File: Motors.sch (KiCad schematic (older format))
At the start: 23 parts, among them J10 Screw_Terminal_01x02, J11 Screw_Terminal_01x02, J12 Screw_Terminal_01x02, J2 MOTOR_1, J3 MOTOR_2, J7 MOTOR_3, J8 MOTOR_4, J9 Screw_Terminal_01x02, U10 TXB0104D, U11 VNH5019, U3 VNH5019, U4 VNH5019, U8 TXB0104D, U9 VNH5019

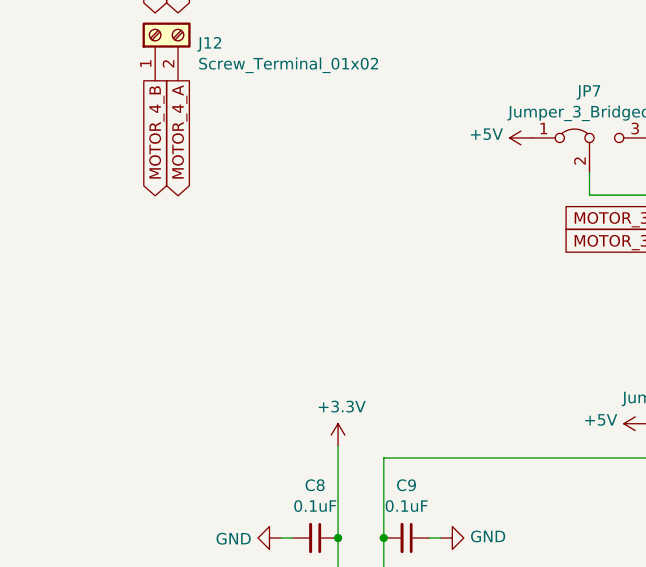
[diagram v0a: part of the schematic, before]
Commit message: Rev B
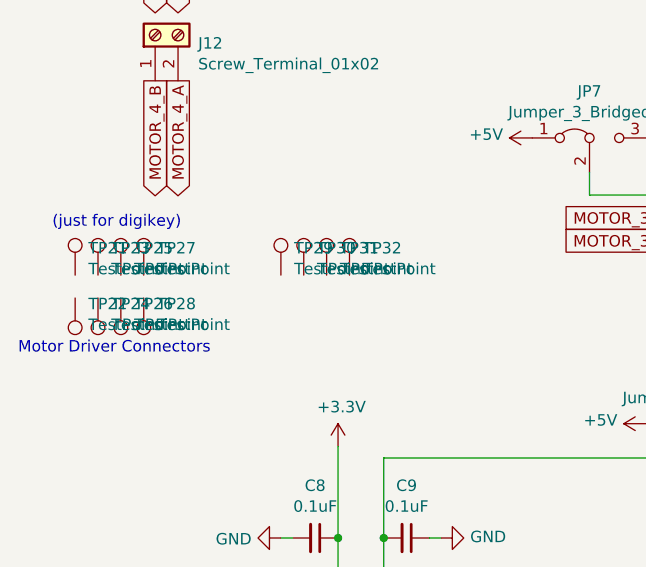
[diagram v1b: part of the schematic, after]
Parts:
- added TP21, TP22, TP23, TP24, TP25, TP26, TP27, TP28, TP29, TP30, TP31, TP32: TestPoint, symbol Connector:TestPoint
- C10, C11, C8, C9: DigiKey (none) -> 399-1100-1-ND
- J10, J11, J12, J9: DigiKey (none) -> 277-1247-ND
- U10, U8: DigiKey (none) -> 296-21928-1-ND
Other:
- note added: "(just for digikey)"
- note added: "Motor Driver Connectors"
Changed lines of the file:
@@
 F 2 "Package_SO:SOIC-14_3.9x8.7mm_P1.27mm" H 2100 5750 50  0001 C CNN
 F 3 "http://www.ti.com/lit/ds/symlink/txb0104.pdf" H 2210 6595 50  0001 C CNN
+F 4 "296-21928-1-ND" H 2100 6500 50  0001 C CNN "DigiKey"
 	1    2100 6500
 	1    0    0    -1
@@
 F 2 "Capacitor_SMD:C_0603_1608Metric_Pad1.05x0.95mm_HandSolder" H 1900 5650 50  0001 C CNN
 F 3 "~" H 1900 5650 50  0001 C CNN
+F 4 "399-1100-1-ND" H 1900 5650 50  0001 C CNN "DigiKey"
 	1    1900 5650
 	0    1    1    0
@@
 F 2 "Capacitor_SMD:C_0603_1608Metric_Pad1.05x0.95mm_HandSolder" H 2300 5650 50  0001 C CNN
 F 3 "~" H 2300 5650 50  0001 C CNN
+F 4 "399-1100-1-ND" H 2300 5650 50  0001 C CNN "DigiKey"
 	1    2300 5650
 	0    1    1    0
@@
 F 2 "Package_SO:SOIC-14_3.9x8.7mm_P1.27mm" H 5050 5750 50  0001 C CNN
 F 3 "http://www.ti.com/lit/ds/symlink/txb0104.pdf" H 5160 6595 50  0001 C CNN
+F 4 "296-21928-1-ND" H 5050 6500 50  0001 C CNN "DigiKey"
 	1    5050 6500
 	1    0    0    -1
@@
 F 2 "Capacitor_SMD:C_0603_1608Metric_Pad1.05x0.95mm_HandSolder" H 4850 5650 50  0001 C CNN
 F 3 "~" H 4850 5650 50  0001 C CNN
+F 4 "399-1100-1-ND" H 4850 5650 50  0001 C CNN "DigiKey"
 	1    4850 5650
 	0    1    1    0
@@
 F 2 "Capacitor_SMD:C_0603_1608Metric_Pad1.05x0.95mm_HandSolder" H 5250 5650 50  0001 C CNN
 F 3 "~" H 5250 5650 50  0001 C CNN
+F 4 "399-1100-1-ND" H 5250 5650 50  0001 C CNN "DigiKey"
 	1    5250 5650
 	0    1    1    0
@@
 F 2 "TerminalBlock_Phoenix:TerminalBlock_Phoenix_MKDS-3-2-5.08_1x02_P5.08mm_Horizontal" H 1200 1050 50  0001 C CNN
 F 3 "~" H 1200 1050 50  0001 C CNN
+F 4 "277-1247-ND" H 1200 1050 50  0001 C CNN "DigiKey"
 	1    1200 1050
 	0    -1   -1   0
@@
 F 2 "TerminalBlock_Phoenix:TerminalBlock_Phoenix_MKDS-3-2-5.08_1x02_P5.08mm_Horizontal" H 1200 1850 50  0001 C CNN
 F 3 "~" H 1200 1850 50  0001 C CNN
+F 4 "277-1247-ND" H 1200 1850 50  0001 C CNN "DigiKey"
 	1    1200 1850
 	0    -1   -1   0
@@
 F 2 "TerminalBlock_Phoenix:TerminalBlock_Phoenix_MKDS-3-2-5.08_1x02_P5.08mm_Horizontal" H 1200 2650 50  0001 C CNN
 F 3 "~" H 1200 2650 50  0001 C CNN
+F 4 "277-1247-ND" H 1200 2650 50  0001 C CNN "DigiKey"
 	1    1200 2650
 	0    -1   -1   0
@@
 F 2 "TerminalBlock_Phoenix:TerminalBlock_Phoenix_MKDS-3-2-5.08_1x02_P5.08mm_Horizontal" H 1200 3450 50  0001 C CNN
 F 3 "~" H 1200 3450 50  0001 C CNN
+F 4 "277-1247-ND" H 1200 3450 50  0001 C CNN "DigiKey"
 	1    1200 3450
 	0    -1   -1   0
@@
 Wire Wire Line
 	2200 5300 2200 5650
+$Comp
+L Connector:TestPoint TP21
+U 1 1 5EF090F9
+P 850 4500
+F 0 "TP21" H 908 4618 50  0000 L CNN
+F 1 "TestPoint" H 908 4527 50  0000 L CNN
+F 2 "" H 1050 4500 50  0001 C CNN
+F 3 "~" H 1050 4500 50  0001 C CNN
+F 4 "S7043-ND" H 850 4500 50  0001 C CNN "DigiKey"
+	1    850  4500
+	1    0    0    -1
+$EndComp
+$Comp
+L Connector:TestPoint TP23
+U 1 1 5EF09D1C
+P 950 4500
+F 0 "TP23" H 1008 4618 50  0000 L CNN
+F 1 "TestPoint" H 1008 4527 50  0000 L CNN
+F 2 "" H 1150 4500 50  0001 C CNN
+F 3 "~" H 1150 4500 50  0001 C CNN
+F 4 "S7043-ND" H 950 4500 50  0001 C CNN "DigiKey"
+	1    950  4500
+	1    0    0    -1
+$EndComp
+$Comp
+L Connector:TestPoint TP25
+U 1 1 5EF09F5F
+P 1050 4500
+F 0 "TP25" H 1108 4618 50  0000 L CNN
+F 1 "TestPoint" H 1108 4527 50  0000 L CNN
+F 2 "" H 1250 4500 50  0001 C CNN
+F 3 "~" H 1250 4500 50  0001 C CNN
+F 4 "S7043-ND" H 1050 4500 50  0001 C CNN "DigiKey"
+	1    1050 4500
+	1    0    0    -1
+$EndComp
+$Comp
+L Connector:TestPoint TP27
+U 1 1 5EF0A180
+P 1150 4500
+F 0 "TP27" H 1208 4618 50  0000 L CNN
+F 1 "TestPoint" H 1208 4527 50  0000 L CNN
+F 2 "" H 1350 4500 50  0001 C CNN
+F 3 "~" H 1350 4500 50  0001 C CNN
+F 4 "S7043-ND" H 1150 4500 50  0001 C CNN "DigiKey"
+	1    1150 4500
+	1    0    0    -1
+$EndComp
+$Comp
+L Connector:TestPoint TP22
+U 1 1 5EF0A47F
+P 850 4600
+F 0 "TP22" H 792 4626 50  0000 R CNN
+F 1 "TestPoint" H 792 4717 50  0000 R CNN
+F 2 "" H 1050 4600 50  0001 C CNN
+F 3 "~" H 1050 4600 50  0001 C CNN
+F 4 "S7041-ND" H 850 4600 50  0001 C CNN "DigiKey"
+	1    850  4600
+	-1   0    0    1
+$EndComp
+$Comp
+L Connector:TestPoint TP24
+U 1 1 5EF0AFA3
+P 950 4600
+F 0 "TP24" H 892 4626 50  0000 R CNN
+F 1 "TestPoint" H 892 4717 50  0000 R CNN
+F 2 "" H 1150 4600 50  0001 C CNN
+F 3 "~" H 1150 4600 50  0001 C CNN
+F 4 "S7041-ND" H 950 4600 50  0001 C CNN "DigiKey"
+	1    950  4600
+	-1   0    0    1
+$EndComp
+$Comp
+L Connector:TestPoint TP26
+U 1 1 5EF0B292
+P 1050 4600
+F 0 "TP26" H 992 4626 50  0000 R CNN
+F 1 "TestPoint" H 992 4717 50  0000 R CNN
+F 2 "" H 1250 4600 50  0001 C CNN
+F 3 "~" H 1250 4600 50  0001 C CNN
+F 4 "S7041-ND" H 1050 4600 50  0001 C CNN "DigiKey"
+	1    1050 4600
+	-1   0    0    1
+$EndComp
+$Comp
+L Connector:TestPoint TP28
+U 1 1 5EF0BE5F
+P 1150 4600
+F 0 "TP28" H 1092 4626 50  0000 R CNN
+F 1 "TestPoint" H 1092 4717 50  0000 R CNN
+F 2 "" H 1350 4600 50  0001 C CNN
+F 3 "~" H 1350 4600 50  0001 C CNN
+F 4 "S7041-ND" H 1150 4600 50  0001 C CNN "DigiKey"
+	1    1150 4600
+	-1   0    0    1
+$EndComp
+Text Notes 750  4300 0    50   ~ 0
+(just for digikey)
+Text Notes 600  4850 0    50   ~ 0
+Motor Driver Connectors
+$Comp
+L Connector:TestPoint TP29
+U 1 1 5EF0E1D1
+P 1750 4500
+F 0 "TP29" H 1808 4618 50  0000 L CNN
+F 1 "TestPoint" H 1808 4527 50  0000 L CNN
+F 2 "" H 1950 4500 50  0001 C CNN
+F 3 "~" H 1950 4500 50  0001 C CNN
+F 4 "S7004-ND" H 1750 4500 50  0001 C CNN "DigiKey"
+	1    1750 4500
+	1    0    0    -1
+$EndComp
+$Comp
+L Connector:TestPoint TP30
+U 1 1 5EF16CF5
+P 1850 4500
+F 0 "TP30" H 1908 4618 50  0000 L CNN
+F 1 "TestPoint" H 1908 4527 50  0000 L CNN
+F 2 "" H 2050 4500 50  0001 C CNN
+F 3 "~" H 2050 4500 50  0001 C CNN
+F 4 "S7004-ND" H 1850 4500 50  0001 C CNN "DigiKey"
+	1    1850 4500
+	1    0    0    -1
+$EndComp
+$Comp
+L Connector:TestPoint TP31
+U 1 1 5EF16FB4
+P 1950 4500
+F 0 "TP31" H 2008 4618 50  0000 L CNN
+F 1 "TestPoint" H 2008 4527 50  0000 L CNN
+F 2 "" H 2150 4500 50  0001 C CNN
+F 3 "~" H 2150 4500 50  0001 C CNN
+F 4 "S7004-ND" H 1950 4500 50  0001 C CNN "DigiKey"
+	1    1950 4500
+	1    0    0    -1
+$EndComp
+$Comp
+L Connector:TestPoint TP32
+U 1 1 5EF172C1
+P 2050 4500
+F 0 "TP32" H 2108 4618 50  0000 L CNN
+F 1 "TestPoint" H 2108 4527 50  0000 L CNN
+F 2 "" H 2250 4500 50  0001 C CNN
+F 3 "~" H 2250 4500 50  0001 C CNN
+F 4 "S7004-ND" H 2050 4500 50  0001 C CNN "DigiKey"
+	1    2050 4500
+	1    0    0    -1
+$EndComp
 $EndSCHEMATC
